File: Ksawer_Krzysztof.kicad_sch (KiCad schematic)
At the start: 57 parts, among them J1 BAT, J3 V1, K1 1461103-1, K2 1461103-1, Q1 BC547, Q2 MMBT3904, Q3 MMBT3904, U1 DHT11, U2 ESP-12E, U3 NHD-C0220BIZ, U4 LTV-844, U5 STM32F038K6Ux, U6 TPS63021DSJR, U8 INA180A1, Y1 ABM3-B.000MHZ-D2Y

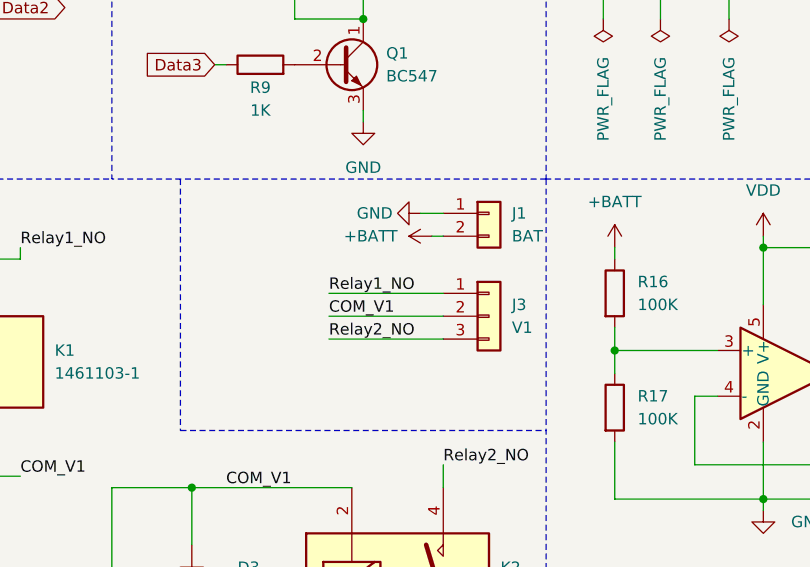
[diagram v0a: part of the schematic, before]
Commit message: zmiana4
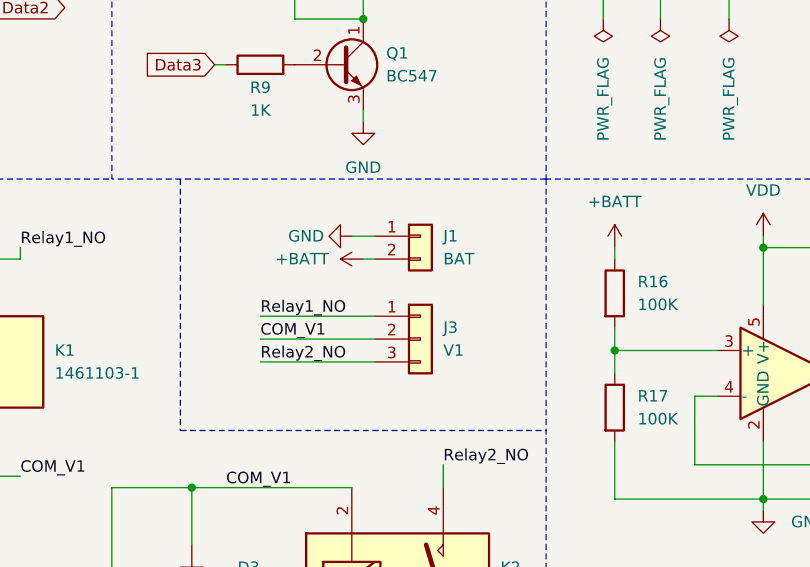
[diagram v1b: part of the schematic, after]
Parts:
- BZ1: footprint (none) -> Buzzer_Beeper:Buzzer_12x9.5RM7.6
- C1, C10, C11, C12, C13, C14, C15, C16, C17, C18, C2, C3, C4, C5, C6, C7, C8, C9: footprint (none) -> Capacitor_SMD:C_0603_1608Metric_Pad1.08x0.95mm_HandSolder
- J1: footprint (none) -> Connector_PinHeader_1.00mm:PinHeader_1x02_P1.00mm_Vertical
- J3: footprint (none) -> Connector_PinHeader_1.00mm:PinHeader_1x03_P1.00mm_Vertical
- L1: footprint (none) -> Inductor_SMD:L_0603_1608Metric
- R1, R10, R11, R12, R13, R14, R15, R16, R17, R18, R2, R3, R4, R5, R7, R8, R9: footprint (none) -> Resistor_SMD:R_0805_2012Metric
- Y1: footprint (none) -> Crystal:Crystal_SMD_5032-2Pin_5.0x3.2mm
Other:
- moved on the sheet: J1, J3
